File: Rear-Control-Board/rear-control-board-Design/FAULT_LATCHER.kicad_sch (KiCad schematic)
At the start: 13 parts, among them J4 JST-B2B-VERT-2PIN, J5 JST-B2B-VERT-2PIN, K2 G5V-2, K3 G5V-2, Q1 2N7002

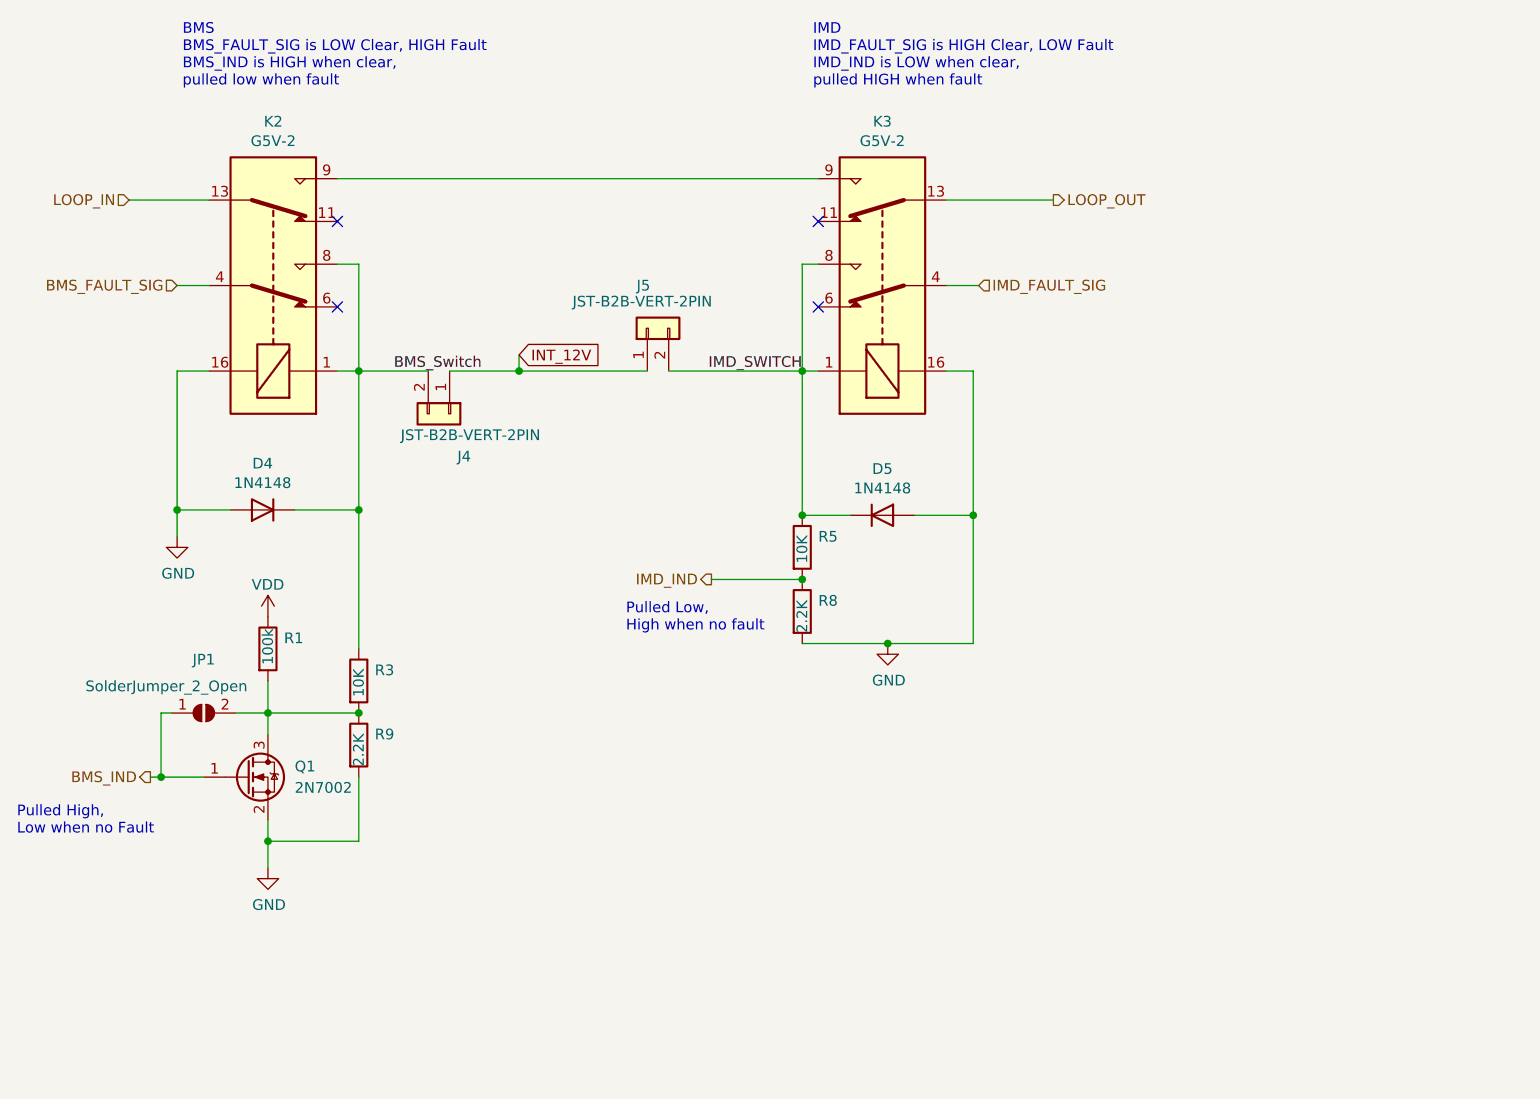
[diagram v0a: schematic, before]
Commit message: end of year DUMP
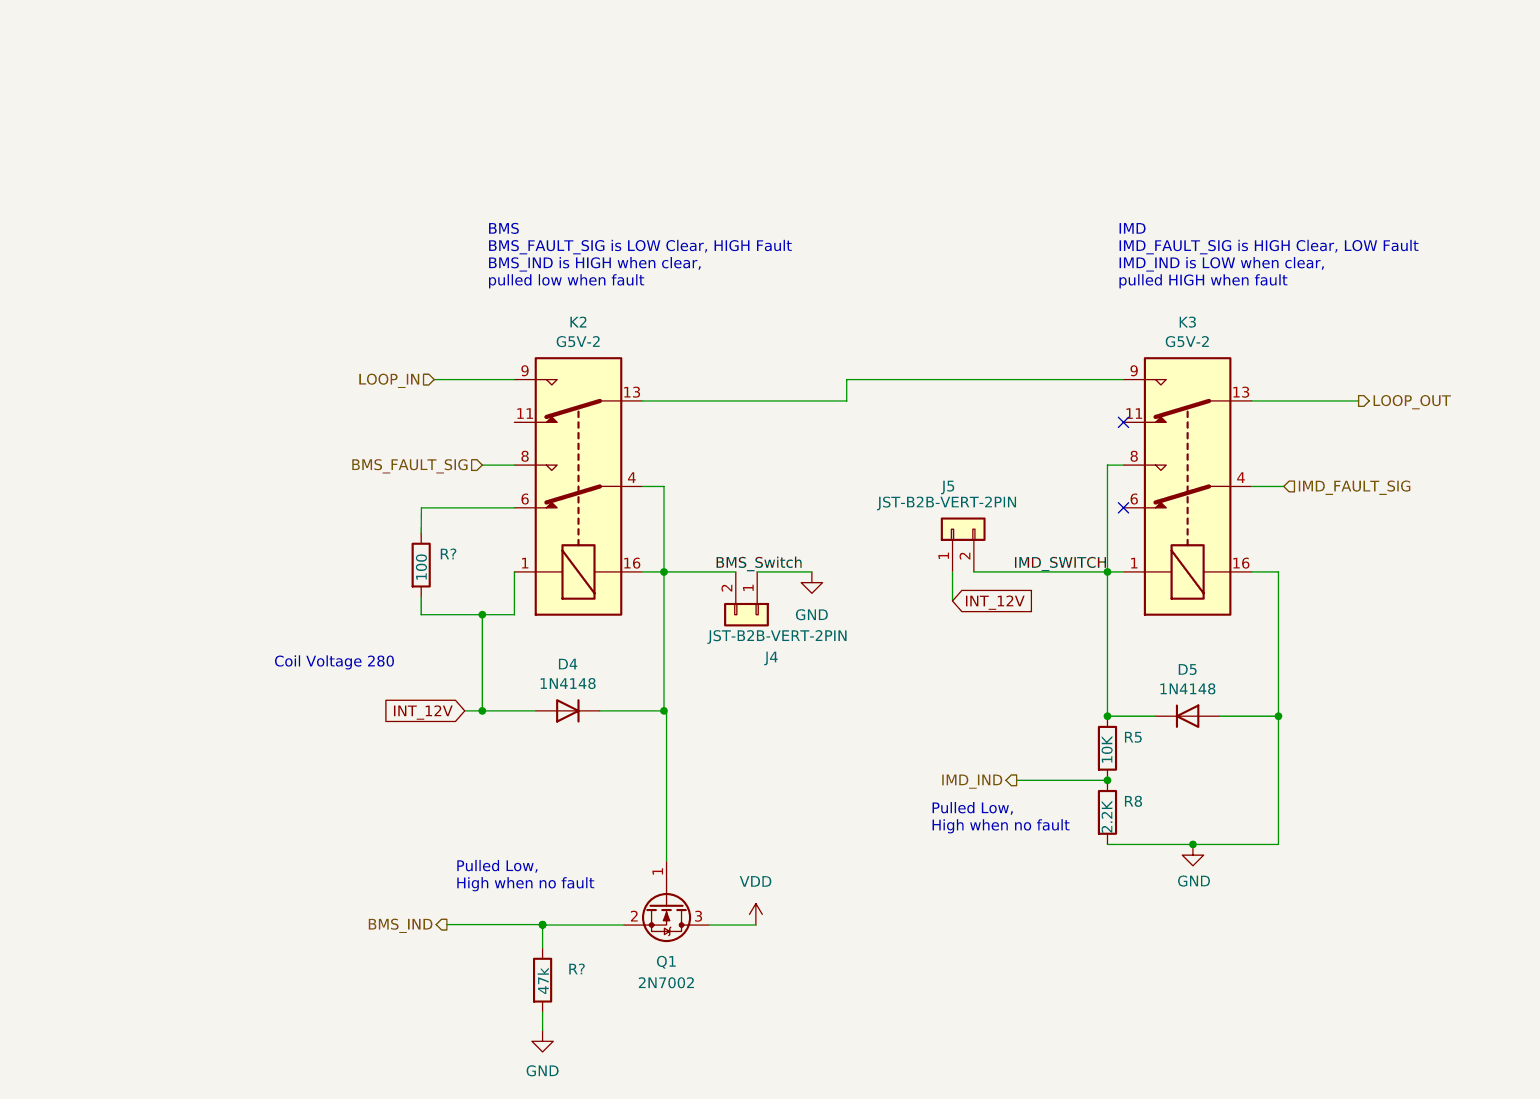
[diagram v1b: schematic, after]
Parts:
- removed JP1: SolderJumper_2_Open, Jumper:SolderJumper-2_P1.3mm_Open_TrianglePad1.0x1.5mm, symbol Jumper:SolderJumper_2_Open
- removed R1: 100k, Resistor_SMD:R_0603_1608Metric_Pad0.98x0.95mm_HandSolder, symbol Device:R
- removed R3: 10K, Resistor_SMD:R_0603_1608Metric_Pad0.98x0.95mm_HandSolder, symbol Device:R
- removed R9: 2.2K, Resistor_SMD:R_0603_1608Metric_Pad0.98x0.95mm_HandSolder, symbol Device:R
- added R?: 47k, symbol Device:R
- added R?: 100, symbol Device:R
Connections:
- net BMS_FAULT_SIG: now also K2.8; no longer K2.4
- net BMS_IND: now also Q1.2 (S), R?.1; no longer Q1.1 (G)
- net GND: now also J4.1 (Pin_1), R?.2; no longer D4.2 (A), K2.16, Q1.2 (S)
- net INT_12V: now also D4.2 (A), K2.1, R?.2; no longer J4.1 (Pin_1)
- net LOOP_IN: now also K2.9; no longer K2.13
- net VDD: now also Q1.3 (D)
- net at D4.1 (K), J4.2 (Pin_2): now also K2.16, K2.4, Q1.1 (G); no longer K2.1, K2.8
- net at K2.6: now also R?.1
- net at K3.9: now also K2.13; no longer K2.9
- no-connect marks 4 -> 2
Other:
- note added: "Coil Voltage 280"
- note removed: "Pulled High, Low when no Fault"
- moved on the sheet: D4, D5, J4, J5, K2, K3, Q1, R5, R8
